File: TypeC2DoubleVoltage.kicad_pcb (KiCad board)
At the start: 2 copper layers, 71.1 x 30.5 mm, 57 parts, among them J1 USB_C_Receptacle_PowerOnly_6P, J2 Conn_01x10_Pin, U1 MC34063AD, U2 LM317_SOT-223, U3 MC34063AD, U4 LM337_SOT223

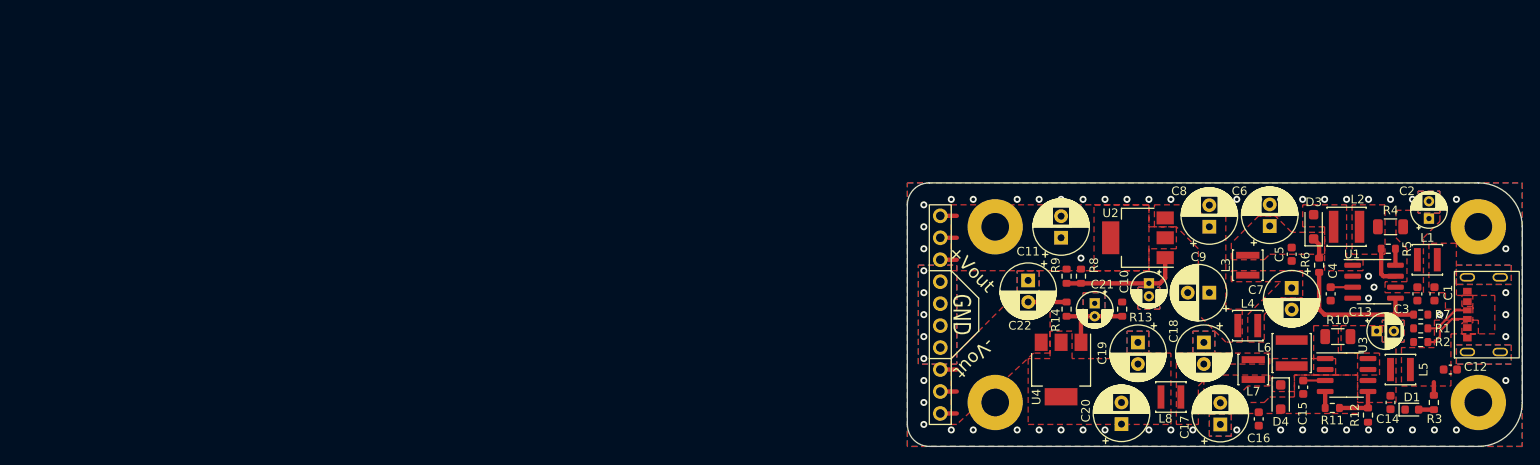
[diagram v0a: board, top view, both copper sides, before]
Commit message: Update
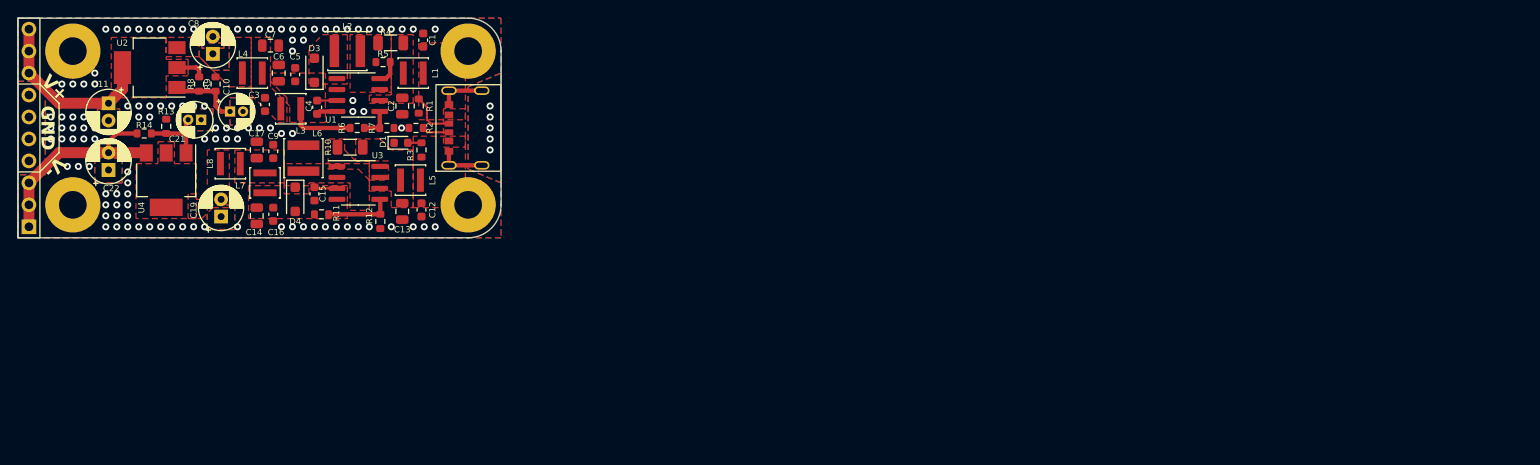
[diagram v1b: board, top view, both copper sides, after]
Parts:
- removed C18, C20: 100uF 16V D6.3xL5, Capacitor_THT:CP_Radial_D6.3mm_P2.50mm
- C11, C19, C22, C8: value 100uF 16V D6.3xL5 -> 47uF 16V D5xL5; footprint Capacitor_THT:CP_Radial_D6.3mm_P2.50mm -> Capacitor_THT:CP_Radial_D5.0mm_P2.00mm
- C13, C2: value 100uF 10V D5xL5 -> 106 0805 25V X5R; footprint Capacitor_THT:CP_Radial_D4.0mm_P2.00mm -> Capacitor_SMD:C_0805_2012Metric
- C14: value 105 0603 25V X5R -> 106 0805 25V X5R; footprint Capacitor_SMD:C_0603_1608Metric -> Capacitor_SMD:C_0805_2012Metric
- C17, C6, C7: value 100uF 16V D6.3xL5 -> 106 0805 25V X5R; footprint Capacitor_THT:CP_Radial_D6.3mm_P2.50mm -> Capacitor_SMD:C_0805_2012Metric
- C9: value 100uF 16V D6.3xL5 -> 105 0603 25V X5R; footprint Capacitor_THT:CP_Radial_D6.3mm_P2.50mm -> Capacitor_SMD:C_0603_1608Metric
- J2: footprint Connector_PinHeader_2.54mm:PinHeader_1x10_P2.54mm_Horizontal -> Connector_PinHeader_2.54mm:PinHeader_1x10_P2.54mm_Vertical
- R10, R4: value 300mR 1206 -> 200mR 1206
- R11, R7: value 1k 0603 -> 499R 0603
- R12, R6: value 10.2k 0603 -> 5.1k 0603
- R13, R9: value 8.25k 0603 -> 5.1k 0603
- R14, R8: value 1k 0603 -> 604R 0603
- moved H2 164.2 mm to (76.5, 99.3)
- moved H1 163.8 mm to (76.5, 81.5)
- moved C3 135.1 mm to (98.7, 87.7)
- moved C14 132.9 mm to (97.8, 100.6), turned to -90 degrees
- moved R7 121.5 mm to (112.8, 90.4)
- moved C7 121.4 mm to (99.4, 80.9), turned to 180 degrees
- moved D1 120.9 mm to (114.5, 92.1)
- moved R3 120.7 mm to (116.8, 93.0), turned to 90 degrees
- moved C1 120.6 mm to (117.0, 80.3), turned to -90 degrees
- moved C12 120.4 mm to (116.8, 99.9), turned to 90 degrees
- moved J1 119.8 mm to (120.0, 90.4)
- moved C2 119.5 mm to (114.6, 87.9)
- moved U1 119.4 mm to (109.5, 86.6)
- moved L1 119.3 mm to (115.9, 84.1)
- moved C4 119.2 mm to (104.8, 88.0)
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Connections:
- C13 pad 1: /U3_Vin -> GNDREF
- C13 pad 2: GNDREF -> /U3_Vin
- C14 pad 1: GNDREF -> /U3_Vout
- C14 pad 2: /U3_Vin -> GNDREF
- C17 pad 1: GNDREF -> Net-(C17-Pad1)
- C17 pad 2: /U3_Vout -> GNDREF
- C2 pad 1: /U1_Vin -> GNDREF
- C2 pad 2: GNDREF -> /U1_Vin
- C3 pad 2: /U1_Vin -> Net-(C3-Pad2)
- C6 pad 1: /U1_Vout -> GNDREF
- C6 pad 2: GNDREF -> /U1_Vout
- C7 pad 1: Net-(C7-Pad1) -> GNDREF
- C7 pad 2: GNDREF -> Net-(C3-Pad2)
- C9 pad 1: /U2_Vin -> Net-(C17-Pad1)
- L3 pad 2: Net-(C7-Pad1) -> Net-(C3-Pad2)
- L4 pad 1: Net-(C7-Pad1) -> Net-(C3-Pad2)
- L7 pad 2: Net-(C18-Pad2) -> Net-(C17-Pad1)
- L8 pad 1: Net-(C18-Pad2) -> Net-(C17-Pad1)
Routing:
- net +12V: track 5.72 -> 24.0 mm
- net -12V: track 10.2 -> 25.1 mm
- net Net-(U1-Vfb): track 17.3 -> 3.68 mm
- net GNDREF: track 0.00 -> 13.2 mm, vias 62 -> 120
- net Net-(U2-ADJ): track 14.0 -> 8.30 mm
- net /U1_Vout: track 2.48 -> 7.75 mm
- net Net-(U1-Ipk): track 4.68 -> 0.00 mm
- net Net-(J1-CC1): track 6.05 -> 3.19 mm
- net Net-(U3-Vfb): track 5.21 -> 7.72 mm
- net /U3_Vout: track 1.91 -> 0.00 mm
- net VCC: track 1.52 -> 0.00 mm
- net Net-(U4-ADJ): track 9.44 -> 7.95 mm
- net Net-(U1-DC): track 1.91 -> 2.82 mm
- added copper zone on B.Cu, net /U2_Vin
- added copper zone on F.Cu, net Net-(C17-Pad1)
- added copper zone on F.Cu, net Net-(C3-Pad2)
- removed copper zone on F.Cu, net -12V
- removed copper zone on F.Cu, net Net-(C18-Pad2)
- removed copper zone on F.Cu, net Net-(C7-Pad1)
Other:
- board size 71.1 x 30.5 mm -> 55.9 x 25.4 mm
- board text added: "V+"
- board text added: "V-"
- board text removed: "+Vout"
- board text removed: "-Vout"
